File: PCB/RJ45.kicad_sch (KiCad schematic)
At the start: 1 part, among them J1 8P8C_Shielded

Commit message: cutout antenna + saved rotation
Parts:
- J1: LCSC (none) -> C386756
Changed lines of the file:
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@@
+			)
+		)
+		(property "LCSC" "C386756"
+			(at 125.73 63.5 0)
+			(effects
+				(font
+					(size 1.27 1.27)
+				)
+				(hide yes)
 			)
 		)

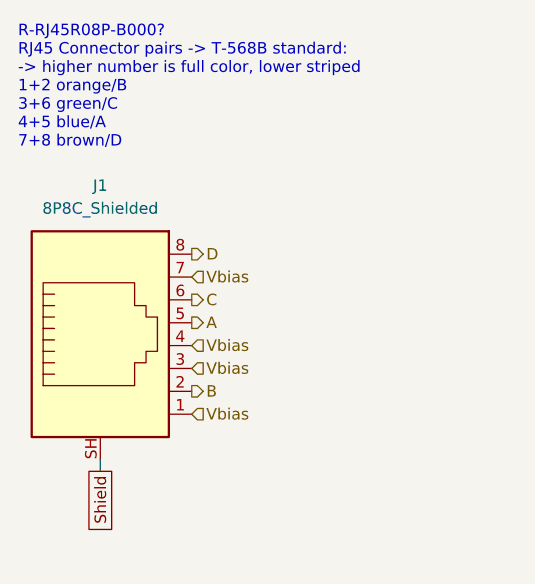
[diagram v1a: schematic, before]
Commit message: prepare for open hardware release
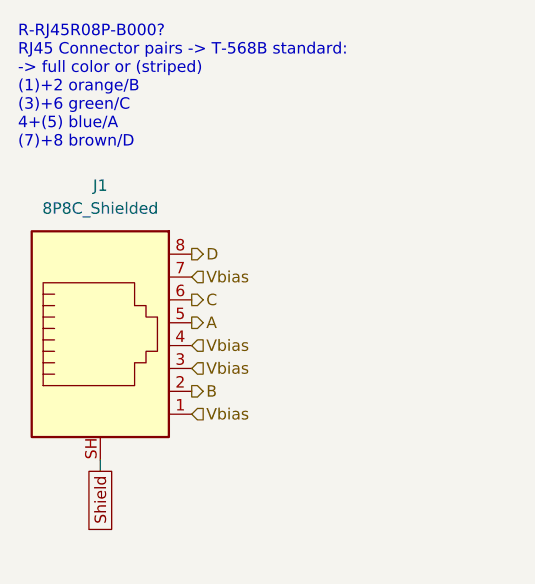
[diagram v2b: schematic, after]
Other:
- note added: "R-RJ45R08P-B000? RJ45 Connector pairs -> T-568B standard: -> full color or (striped) (1)+2 orange/B (3)+6 green/C 4+(5) blue/A (7)+8 brown/D"
- note removed: "R-RJ45R08P-B000? RJ45 Connector pairs -> T-568B standard: -> higher number is full color, lower striped 1+2 orange/B 3+6 green/C 4+5 blue/A 7+8 brown/D"
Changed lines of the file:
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@@
 (kicad_sch
-	(version 20250114)
+	(version 20260306)
 	(generator "eeschema")
-	(generator_version "9.0")
+	(generator_version "10.0")
 	(paper "A4")
-	(text "R-RJ45R08P-B000?\nRJ45 Connector pairs -> T-568B standard:\n-> higher number is full color, lower striped\n1+2 orange/B\n3+6 green/C\n4+5 blue/A\n7+8 brown/D\n"
+	(text "R-RJ45R08P-B000?\nRJ45 Connector pairs -> T-568B standard:\n-> full color or (striped)\n(1)+2 orange/B\n(3)+6 green/C\n4+(5) blue/A\n(7)+8 brown/D\n"
 		(exclude_from_sim no)
 		(at 116.586 52.578 0)
@@
 		(property "Intersheetrefs" "${INTERSHEET_REFS}"
 			(at 125.73 102.99 90)
+			(hide yes)
+			(show_name no)
+			(do_not_autoplace no)
 			(effects
 				(font
@@
 				)
 				(justify right)
-				(hide yes)
 			)
 		)
@@
 		(at 125.73 81.28 0)
 		(unit 1)
+		(body_style 1)
 		(exclude_from_sim no)
 		(in_bom yes)
 		(on_board yes)
+		(in_pos_files yes)
 		(dnp no)
 		(fields_autoplaced yes)
 		(property "Reference" "J1"
 			(at 125.73 63.5 0)
+			(show_name no)
+			(do_not_autoplace no)
 			(effects
 				(font
@@
 		(property "Value" "8P8C_Shielded"
 			(at 125.73 66.04 0)
+			(show_name no)
+			(do_not_autoplace no)
 			(effects
 				(font
@@
 		(property "Footprint" "R-RJ45R08P-B000:R-RJ45R08P-B000"
 			(at 125.73 80.645 90)
-			(effects
-				(font
-					(size 1.27 1.27)
-				)
-				(hide yes)
-			)
-		)
-		(property "Datasheet" "~"
+			(hide yes)
+			(show_name no)
+			(do_not_autoplace no)
+			(effects
+				(font
+					(size 1.27 1.27)
+				)
+			)
+		)
+		(property "Datasheet" ""
 			(at 125.73 80.645 90)
-			(effects
-				(font
-					(size 1.27 1.27)
-				)
-				(hide yes)
+			(hide yes)
+			(show_name no)
+			(do_not_autoplace no)
+			(effects
+				(font
+					(size 1.27 1.27)
+				)
 			)
 		)
 		(property "Description" "RJ connector, 8P8C (8 positions 8 connected), RJ31/RJ32/RJ33/RJ34/RJ35/RJ41/RJ45/RJ49/RJ61, Shielded"
 			(at 125.73 81.28 0)
-			(effects
-				(font
-					(size 1.27 1.27)
-				)
-				(hide yes)
+			(hide yes)
+			(show_name no)
+			(do_not_autoplace no)
+			(effects
+				(font
+					(size 1.27 1.27)
+				)
 			)
 		)
 		(property "LCSC" "C386756"
 			(at 125.73 63.5 0)
-			(effects
-				(font
-					(size 1.27 1.27)
-				)
-				(hide yes)
+			(hide yes)
+			(show_name no)
+			(do_not_autoplace no)
+			(effects
+				(font
+					(size 1.27 1.27)
+				)
 			)
 		)
@@
 		)
 		(instances
-			(project "Schlaubi-Schlumpf"
+			(project "Multi-Ferro-DAQ"
 				(path "/adec948c-82e6-4ad4-8e75-b19e612c0d17/2131c80a-ce05-49b0-92ac-52a13fef390c/adf6e25c-f47c-4ac9-9c2f-f22ac4b1a7f4"
 					(reference "J5")
